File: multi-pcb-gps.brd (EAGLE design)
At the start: 36.5 x 41.9 mm, 8 parts, among them Q1 BS170, X1 6B-ZR

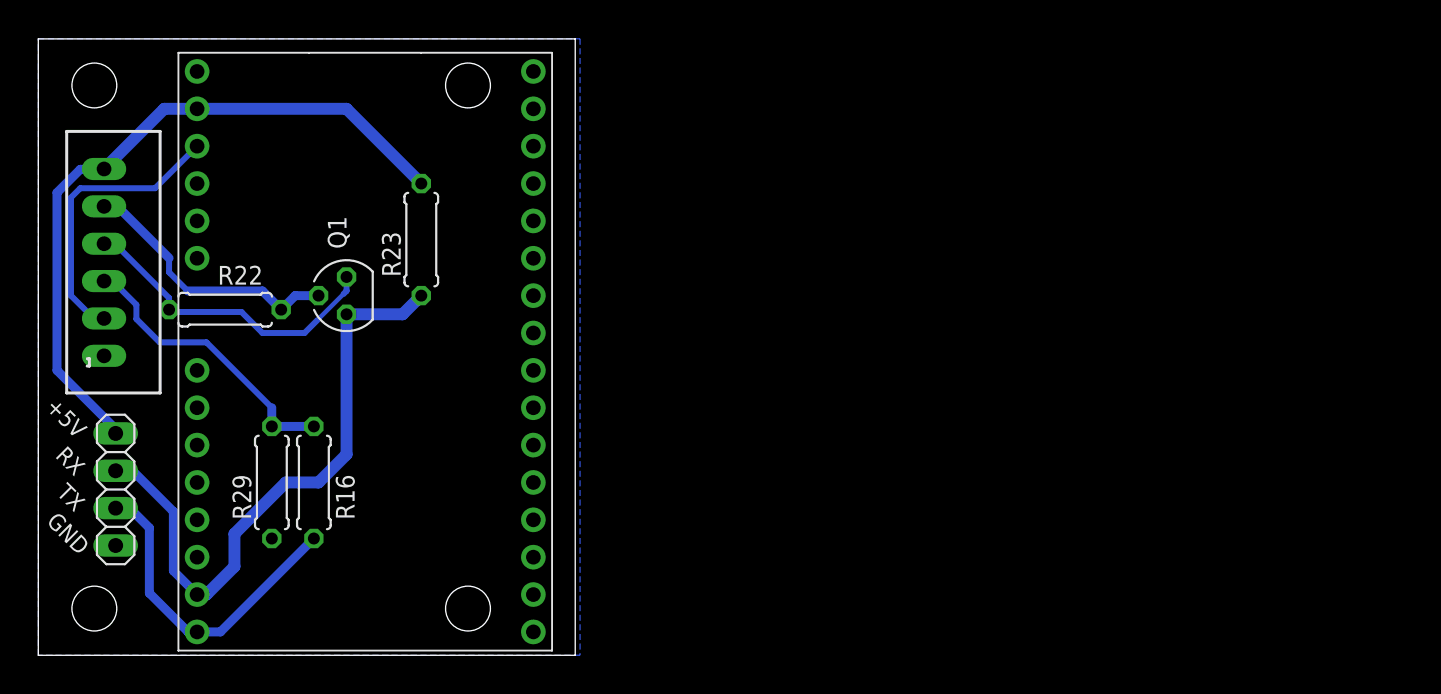
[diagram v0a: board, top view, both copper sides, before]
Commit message: updated some PCB's
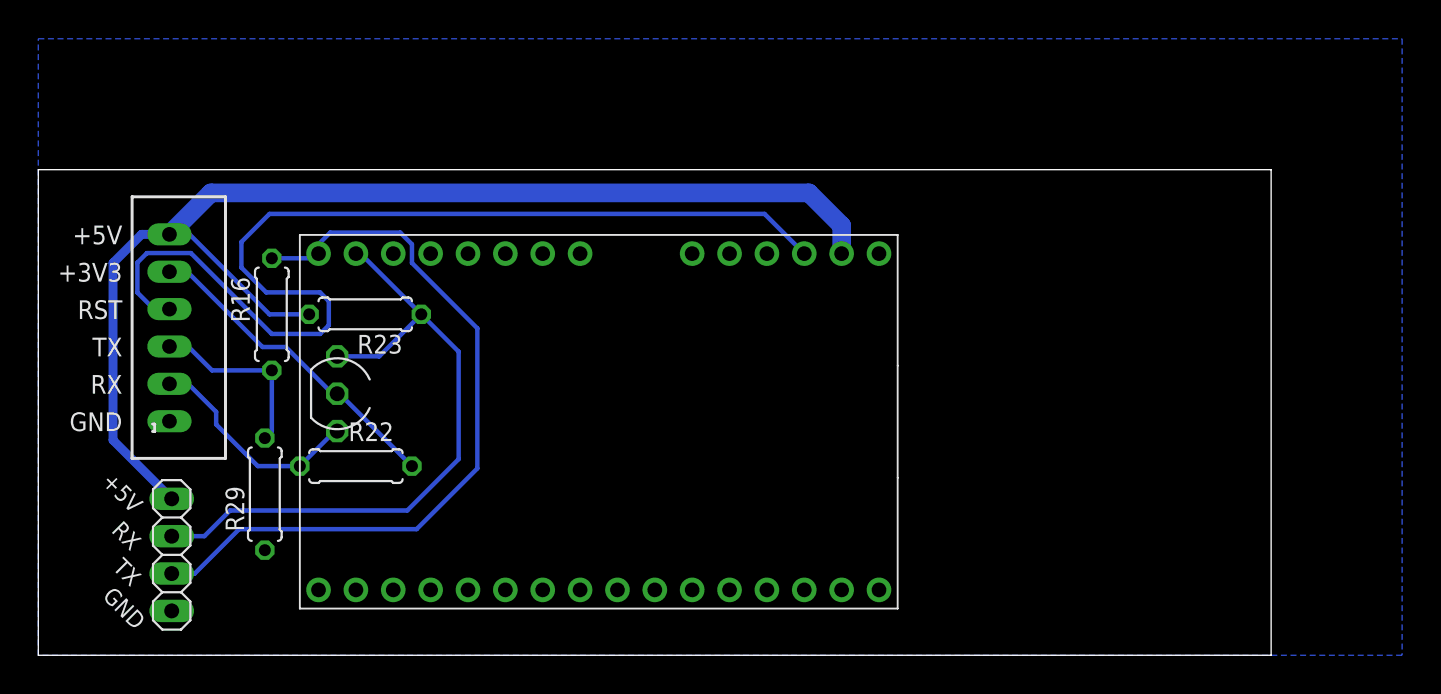
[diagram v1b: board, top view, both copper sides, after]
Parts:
- Q1: value BS170 -> BS170WIDE; device transistor-small-signal:SOT54E -> samuel:SOT54E2
- moved U$6 16.6 mm to (38.1, 15.9), turned to 270 degrees
- moved R22 13.9 mm to (21.6, 12.9)
- moved R16 11.8 mm to (15.9, 23.2), turned to 270 degrees
- moved Q1 6.70 mm to (20.3, 17.8), turned to 270 degrees
- moved R23 6.35 mm to (22.2, 23.2), turned to 180 degrees
- moved X1 6.29 mm to (8.92, 22.3)
- moved JP_UART2 5.85 mm to (9.07, 6.83)
- moved R29 0.93 mm to (15.4, 11.0)
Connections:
- net MCU_RESET: now also X1.4; no longer X1.2
- net UART2_TX: now also X1.2; no longer X1.4
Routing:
- net MCU_RESET: track 19.6 -> 70.9 mm
- net +5V: track 47.3 -> 83.8 mm
- net GPS_TX: track 22.2 -> 51.8 mm
- net UART2_RX: track 19.7 -> 12.4 mm
- net UART2_TX: track 21.6 -> 15.2 mm
- net GPS_RX: track 41.9 -> 45.6 mm
- net +3V3: track 18.4 -> 22.0 mm
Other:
- board size 36.5 x 41.9 mm -> 83.8 x 33 mm
- board text added: "+3V3"
- board text added: "RST"

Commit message: Last iteration of the board
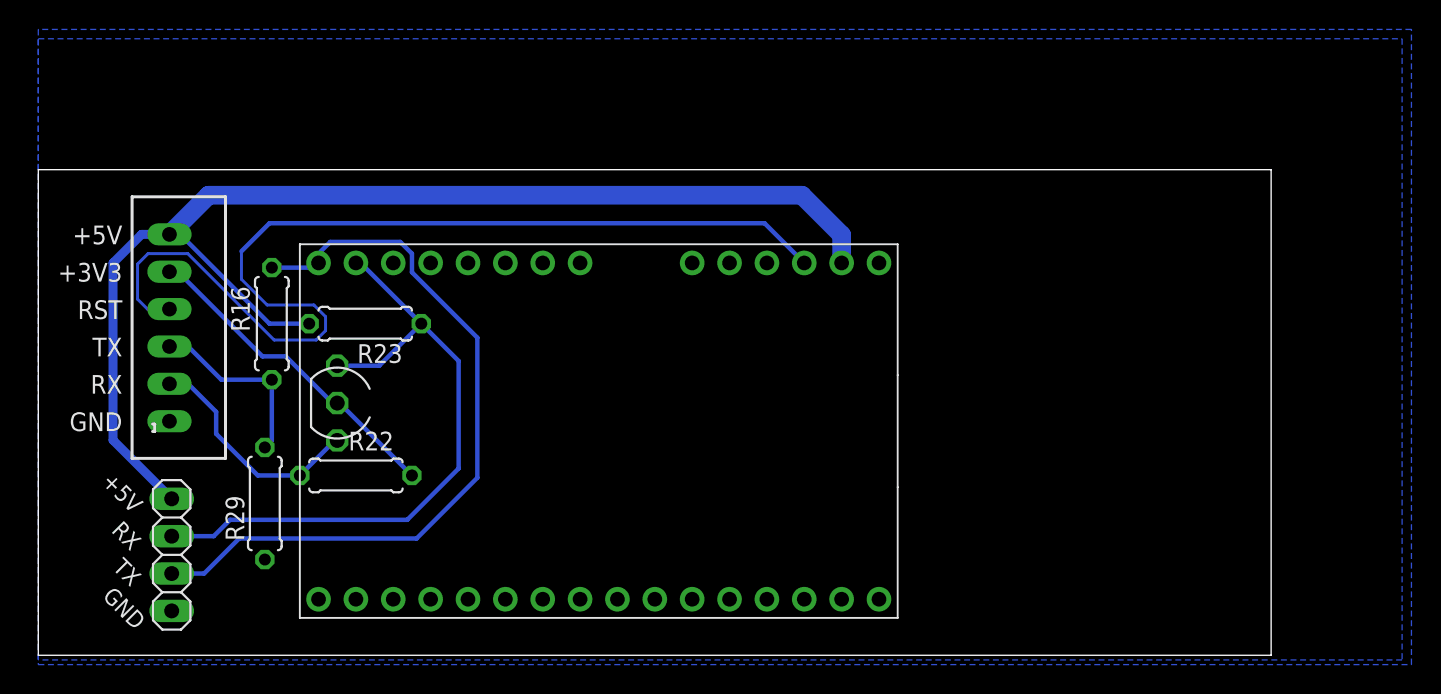
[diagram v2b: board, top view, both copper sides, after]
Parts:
- moved Q1 0.64 mm to (20.3, 17.1)
- moved R22 0.63 mm to (21.6, 12.2)
- moved R29 0.63 mm to (15.4, 10.3)
- moved U$6 0.63 mm to (38.1, 15.2)
- moved R16 0.63 mm to (15.9, 22.5)
- moved R23 0.63 mm to (22.2, 22.5)
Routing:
- net UART2_TX: track 15.2 -> 15.8 mm
